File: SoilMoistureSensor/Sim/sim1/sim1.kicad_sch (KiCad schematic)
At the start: 32 parts, among them U1 74AUC1G86, U10 74AUC1G66, U11 74AUC1G66, U12 74AUC1G66, U2 74AUC1G86, U3 74AUC1G86, U4 74AUC1G86, U5 74AUC1G08, U6 74AUC1G08, U7 OPA356xxDBV, U8 OPA356xxDBV, U9 74AUC1G66

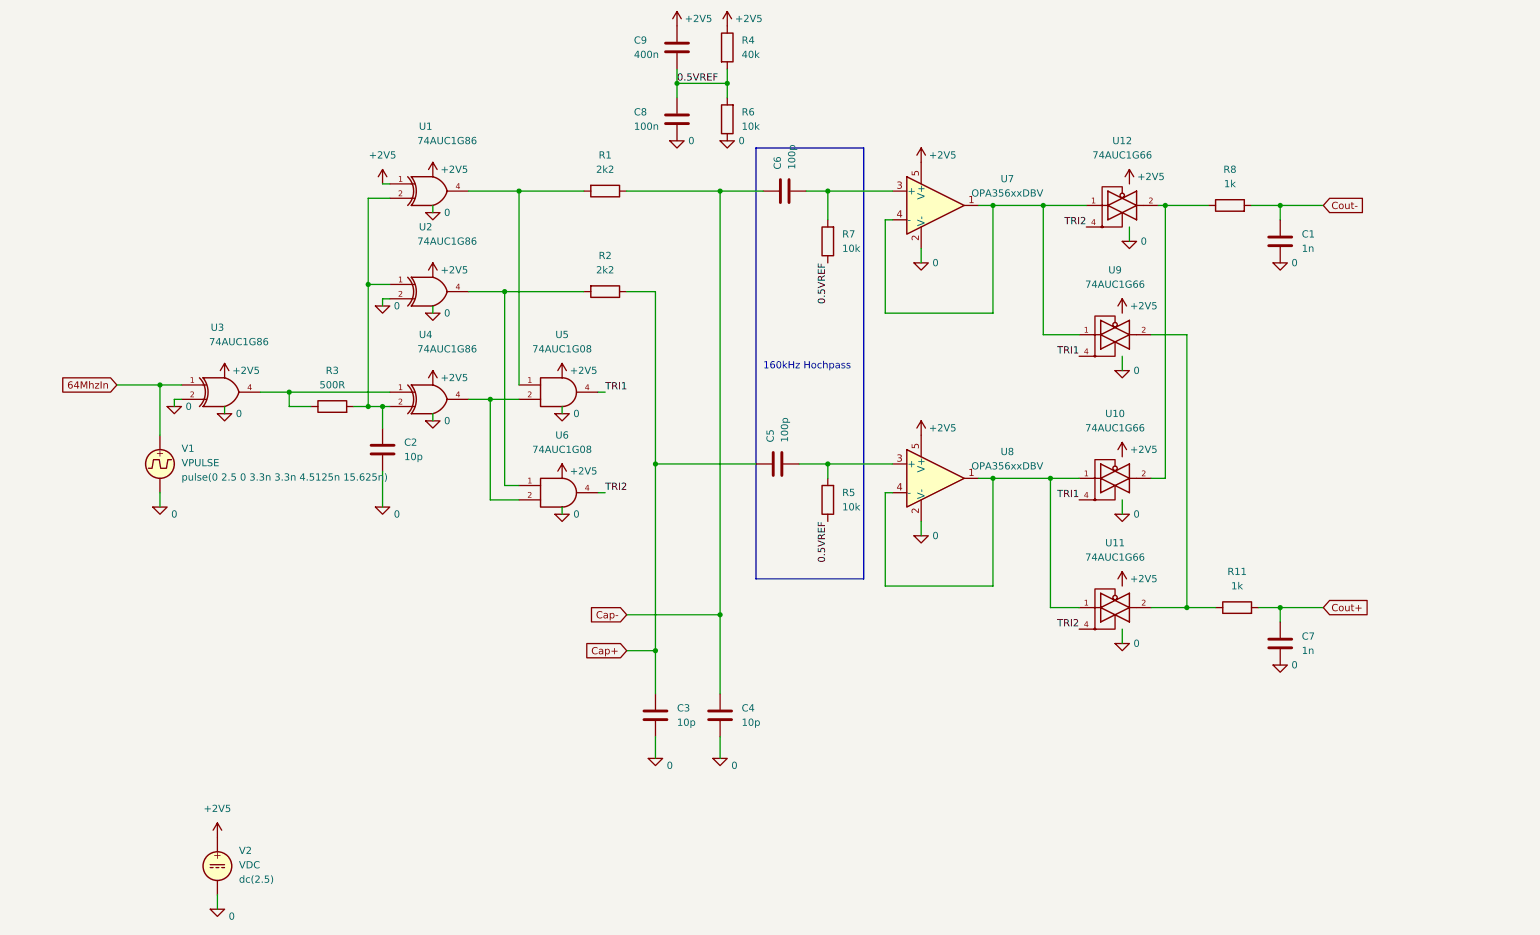
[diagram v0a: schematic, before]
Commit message: - wip
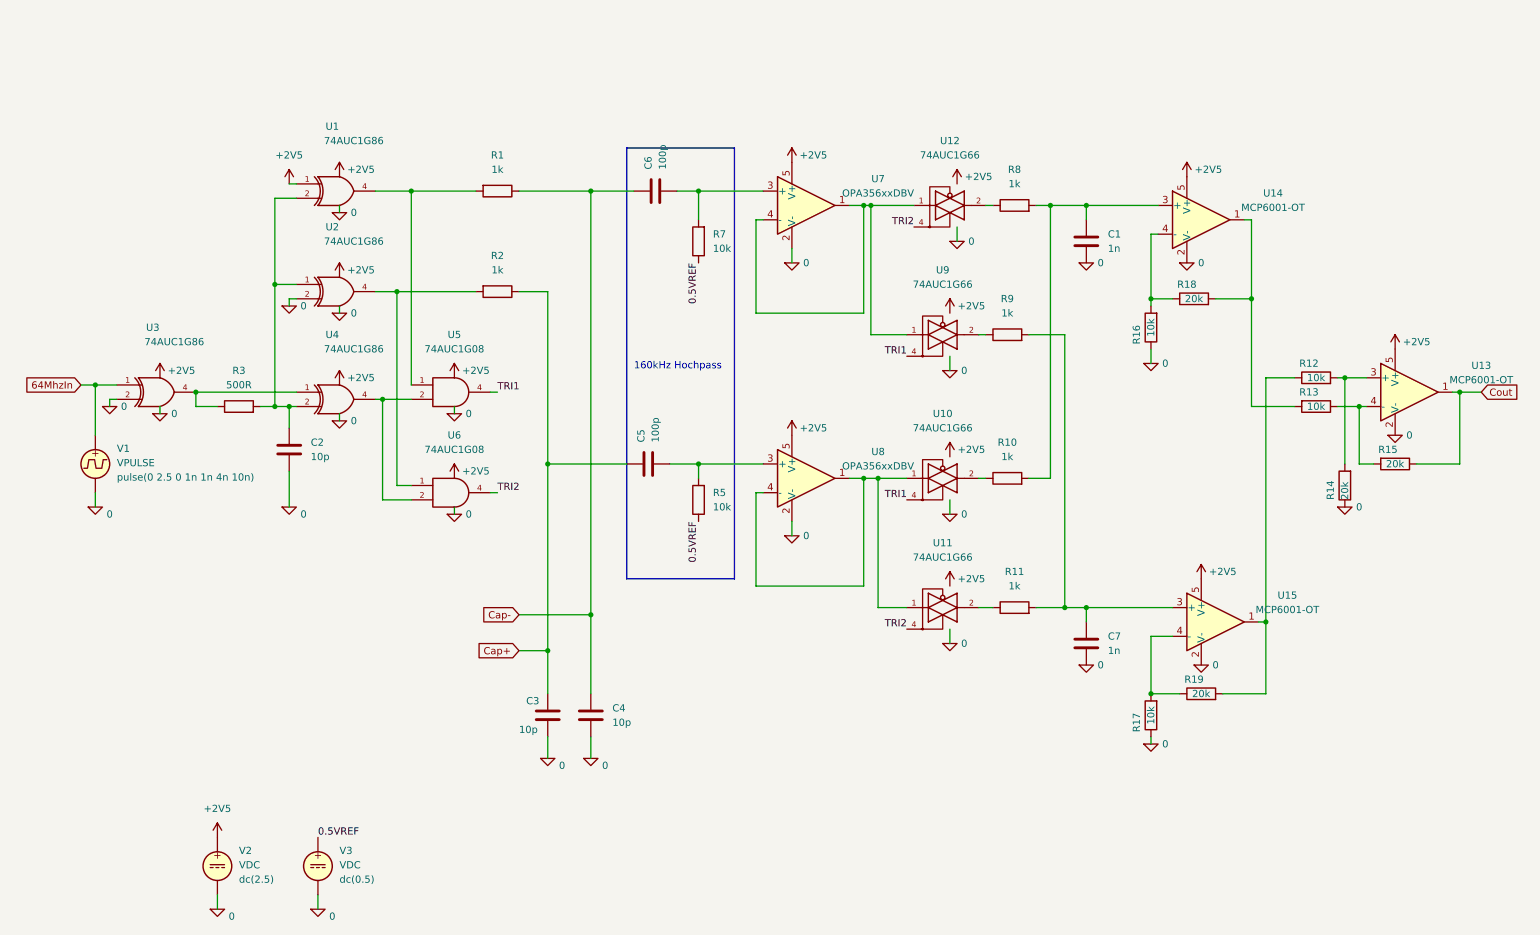
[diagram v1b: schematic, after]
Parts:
- removed C8: 100n, symbol Device:C
- removed C9: 400n, symbol Device:C
- removed R4: 40k, symbol Device:R
- removed R6: 10k, symbol Device:R
- added R10, R9: 1k, symbol Device:R
- added R12, R13, R16, R17: 10k, symbol Device:R
- added R14, R15, R18, R19: 20k, symbol Device:R
- added U13, U14, U15: MCP6001-OT, Package_TO_SOT_SMD:SOT-23-5, symbol Amplifier_Operational:MCP6001-OT
- added V3: VDC, symbol Simulation_SPICE:VDC
- C1: Spice_Model (none) -> 1n; Spice_Netlist_Enabled (none) -> Y; Spice_Primitive (none) -> C
- C3, C4: Spice_Model (none) -> 10p IC=1.25; Spice_Netlist_Enabled (none) -> Y; Spice_Primitive (none) -> C
- R1, R2: value 2k2 -> 1k
- V1: Spice_Model pulse(0 2.5 0 3.3n 3.3n 4.5125n 15.625n) -> pulse(0 2.5 0 1n 1n 4n 10n)
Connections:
- net +2V5: now also U13.5 (V+), U14.5 (V+), U15.5 (V+)
- net 0: now also R14.1, R16.1, R17.1, U13.2 (V-), U14.2 (V-), U15.2 (V-), V3.2
- net 0.5VREF: now also V3.1
- net at R11.1, U11.2: no longer U9.2
- net at R8.1, U12.2: no longer U10.2
- net Cout+: no longer names the net of C7.1, R11.2
- net Cout+: now also R9.2, U15.3 (+)
- net Cout-: no longer names the net of C1.1, R8.2
- net Cout-: now also R10.2, U14.3 (+)
- new net: R13.1, R15.2, U13.4 (-)
- new net: R13.2, R18.2, U14.1
- new net: R9.1, U9.2
- new net: R12.2, R14.2, U13.3 (+)
- new net: R16.2, R18.1, U14.4 (-)
- new net: R10.1, U10.2
- new net: R12.1, R19.2, U15.1
- new net: R17.2, R19.1, U15.4 (-)
- new net Cout: R15.1, U13.1
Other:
- moved on the sheet: C1, C2, C3, C4, C5, C6, C7, R1, R11, R2, R3, R5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
